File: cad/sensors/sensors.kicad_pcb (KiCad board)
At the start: 2 copper layers, 72 x 50 mm, 79 parts, among them J1 Conn_01x04, J2 Conn_01x04, J3 6P6C, J4 Conn_01x04, J5 Conn_01x04, J6 Conn_01x04, J7 Conn_01x02, U1 LMV324, U2 PCA9517A, U3 LMV331, U4 MC14040B, U5 MC14040B, U6 TCA9555DBR, U7 PCF8574

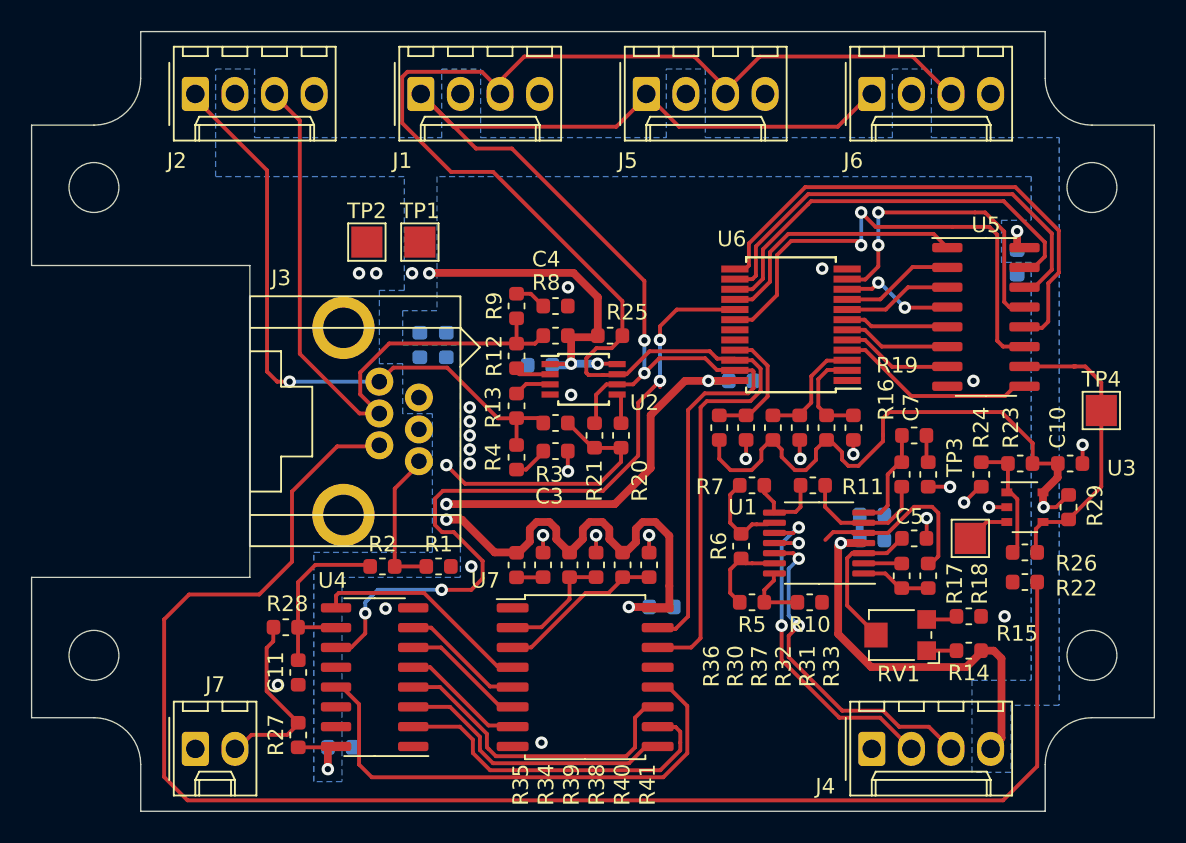
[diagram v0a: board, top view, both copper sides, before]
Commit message: Finished sensor board layout
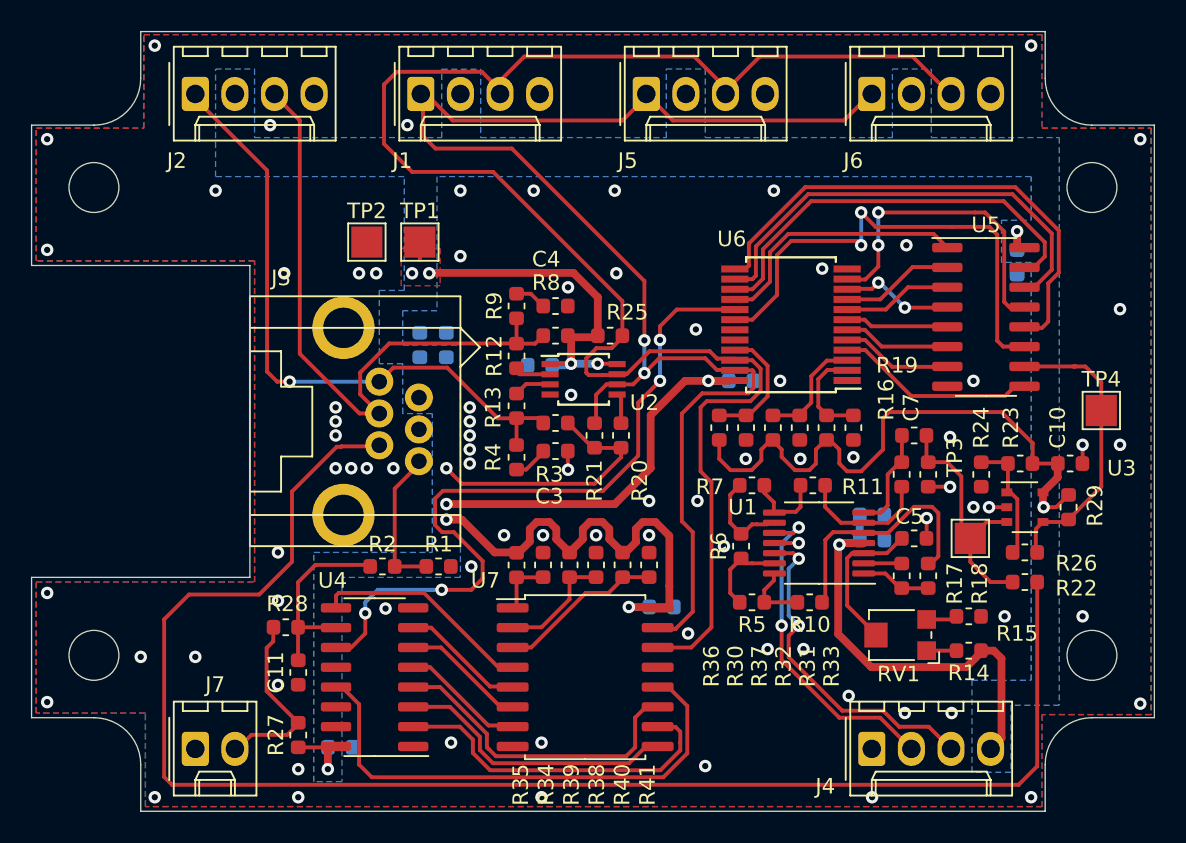
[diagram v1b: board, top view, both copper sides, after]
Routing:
- net Net-(C7-Pad2): track 3.37 -> 14.0 mm
- net GND: track 16.2 -> 8.09 mm, vias 29 -> 80
- net Net-(R10-Pad1): track 11.7 -> 15.5 mm
- net /SCL: track 104.3 -> 107.7 mm
- net Net-(R34-Pad2): track 1.80 -> 3.80 mm
- net /3V3: track 165.8 -> 167.6 mm
- net /SDA: track 92.5 -> 94.1 mm
- net /ADC: track 100.4 -> 99.5 mm
- net (no net): vias 0 -> 3
- added copper zone on F.Cu, net /3V3
- added copper zone on B.Cu, net GND
- added copper zone on F.Cu, net GND
